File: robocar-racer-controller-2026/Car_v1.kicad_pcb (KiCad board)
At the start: 2 copper layers, 92.5 x 119.5 mm, 34 parts, among them J1 GY-87, J10 Buck in, J11 Motor_in, J12 Bateria 3s, J13 Buck_out, J14 Raspbery_usbc, J2 Barramento 16 pinos, J3 Conn_01x03_Pin, J4 Conn_01x03_Pin, J5 Conn_01x19_Socket, J6 Conn_01x19_Socket, J8 ADS1115, J9 Bateria 2s, SW1 SW_DPST_x2, SW2 SW_DPST_x2, U2 ESP32-DEVKITC-32D

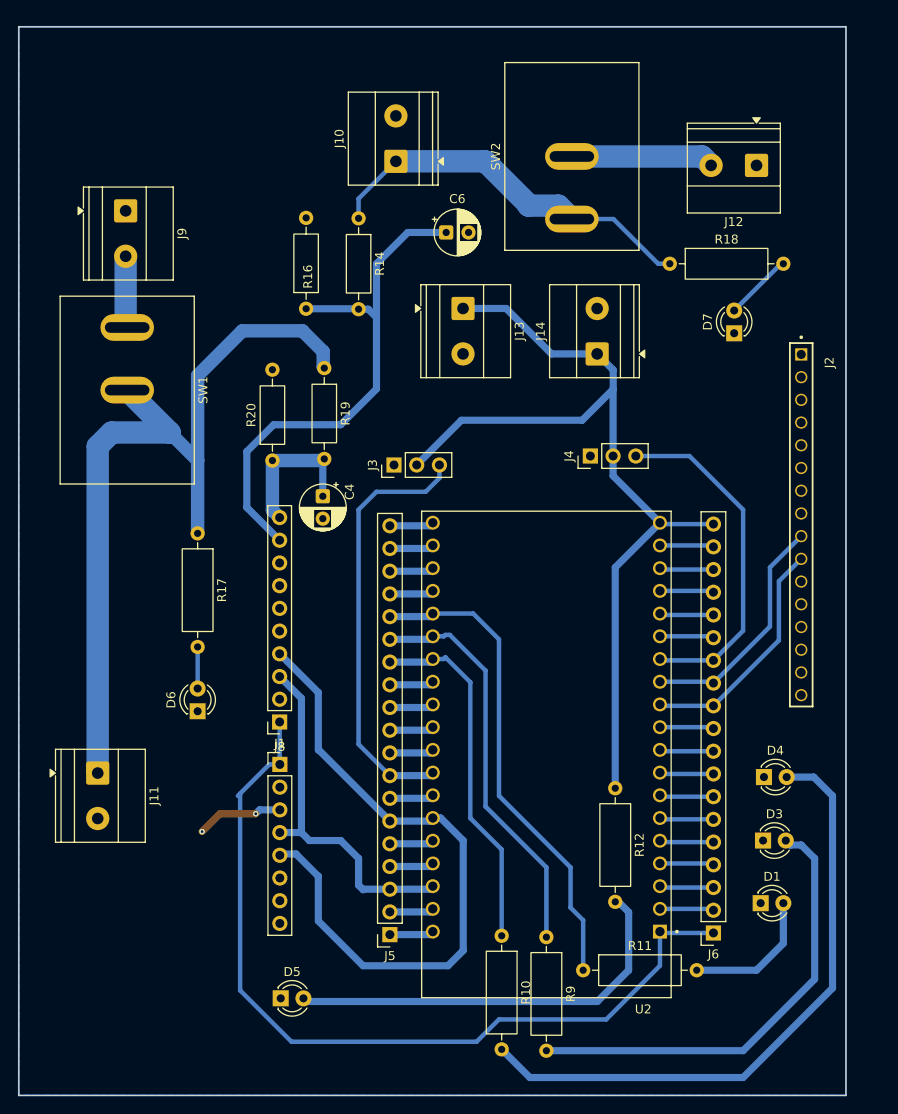
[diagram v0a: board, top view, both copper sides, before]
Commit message: organizando o esquematico
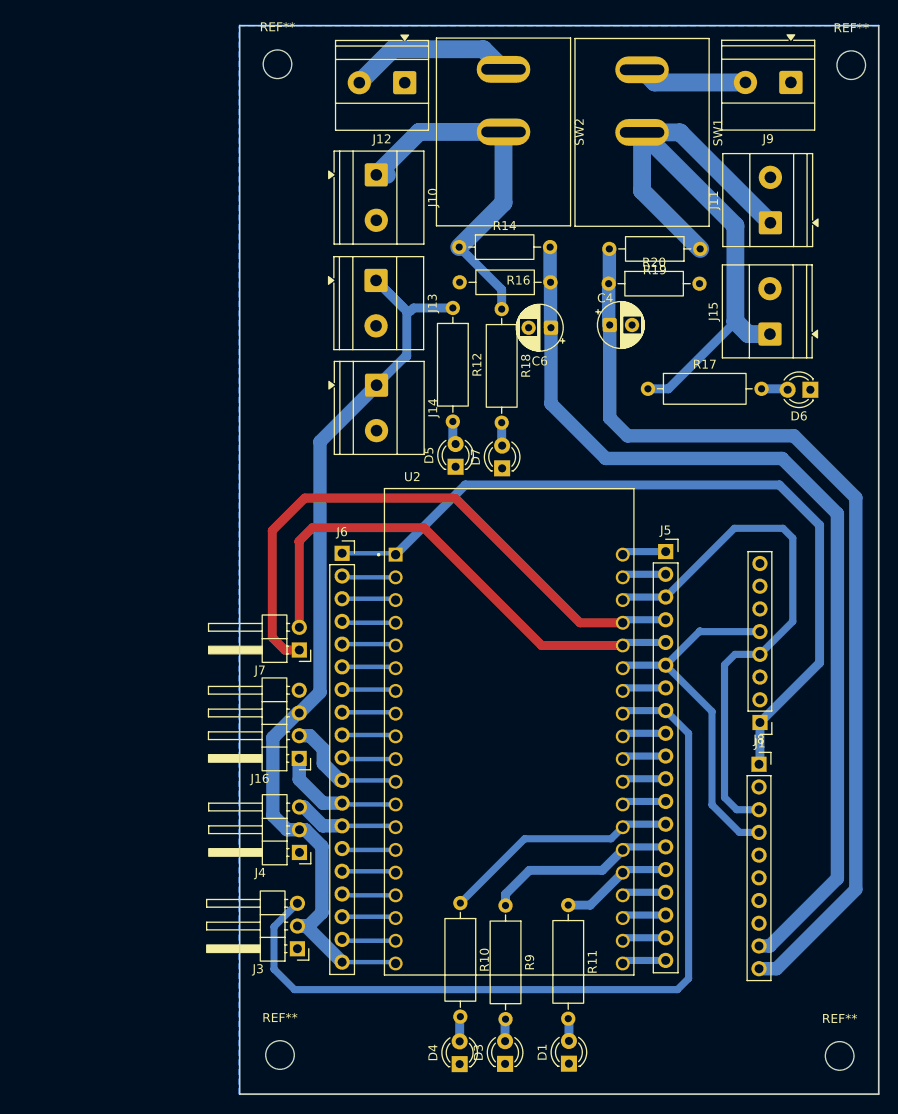
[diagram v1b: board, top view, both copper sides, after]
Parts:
- removed J2: Barramento 16 pinos, Connector:SAMTEC_TSW-116-22-T-S
- added J15: Step_up, TerminalBlock_Phoenix:TerminalBlock_Phoenix_MKDS-1,5-2-5.08_1x02_P5.08mm_Horizontal, F.Cu at (119.0, 81.9)
- added J16: Radio, Connector_PinHeader_2.54mm:PinHeader_1x04_P2.54mm_Horizontal, F.Cu at (66.4, 129.3)
- added J7: Serial, Connector_PinHeader_2.54mm:PinHeader_1x02_P2.54mm_Horizontal, F.Cu at (66.4, 117.2)
- added REF**: MountingHole_3.2mm_M3, MountingHole:MountingHole_3.2mm_M3, F.Cu at (63.9, 51.7)
- added REF**: MountingHole_3.2mm_M3, MountingHole:MountingHole_3.2mm_M3, F.Cu at (64.2, 162.5)
- added REF**: MountingHole_3.2mm_M3, MountingHole:MountingHole_3.2mm_M3, F.Cu at (128.1, 51.8)
- added REF**: MountingHole_3.2mm_M3, MountingHole:MountingHole_3.2mm_M3, F.Cu at (126.8, 162.6)
- J3: value Conn_01x03_Pin -> Sinal_Servo; footprint Connector_PinHeader_2.54mm:PinHeader_1x03_P2.54mm_Vertical -> Connector_PinHeader_2.54mm:PinHeader_1x03_P2.54mm_Horizontal
- J4: value Conn_01x03_Pin -> Sinal_Motor; footprint Connector_PinHeader_2.54mm:PinHeader_1x03_P2.54mm_Vertical -> Connector_PinHeader_2.54mm:PinHeader_1x03_P2.54mm_Horizontal
- moved J11 97.2 mm to (119.1, 69.4), turned to 90 degrees
- moved D6 77.4 mm to (123.5, 88.1), turned to 180 degrees
- moved J9 75.8 mm to (121.3, 53.7), turned to 180 degrees
- moved J6 64.6 mm to (71.2, 152.4), turned to 180 degrees
- moved SW1 64.4 mm to (104.7, 59.3)
- moved D5 62.6 mm to (83.8, 96.7), turned to 90 degrees
- moved J5 58.0 mm to (107.3, 152.2), turned to 180 degrees
- moved R12 56.7 mm to (83.5, 78.9)
- moved J3 55.2 mm to (66.2, 150.6), turned to 180 degrees
- moved J4 55.0 mm to (66.4, 139.8), turned to 180 degrees
- moved J1 53.9 mm to (117.9, 125.3), turned to 180 degrees
- moved J8 53.8 mm to (117.8, 130.0), turned to 0 degrees
- moved R17 52.9 mm to (105.4, 88.0), turned to 0 degrees
- moved D4 46.8 mm to (84.3, 163.5), turned to 90 degrees
- moved R19 44.1 mm to (111.2, 72.3), turned to 180 degrees
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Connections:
- J5 pad 4: /TXD0 -> TX_RASPBERRY
- J5 pad 5: /RXD0 -> RX_RASPBERRY
- SW2 pad 1: +12V -> Net-(J12-Pin_2)
- SW2 pad 2: Net-(J12-Pin_2) -> +12V
- U2 pad J3-4: /TXD0 -> TX_RASPBERRY
- U2 pad J3-5: /RXD0 -> RX_RASPBERRY
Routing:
- net ADC3: track 16.8 -> 108.5 mm
- net Net-(D4-Pad2): track 69.9 -> 2.80 mm
- net TX_RASPBERRY: track 0.00 -> 66.5 mm
- net RX_RASPBERRY: track 0.00 -> 56.4 mm
- net Net-(D3-Pad2): track 50.9 -> 2.48 mm
- net ADC2: track 60.4 -> 107.3 mm
- net Sinal do servo: track 48.1 -> 92.2 mm
- net Net-(D5-Pad2): track 46.6 -> 2.64 mm
- net Estado_1: track 54.4 -> 12.5 mm
- net SDA: track 74.9 -> 41.4 mm
- net Sinal do Motor: track 38.8 -> 11.7 mm
- net Estado_2: track 45.2 -> 21.4 mm
- net SCL: track 39.6 -> 60.5 mm
- net +8V: track 93.0 -> 77.1 mm
- net Estado_3: track 40.2 -> 26.6 mm
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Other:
- board size 92.5 x 119.5 mm -> 71.5 x 119.5 mm
